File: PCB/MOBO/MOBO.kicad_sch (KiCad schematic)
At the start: 17 parts, among them J101 COMP_OUT, J102 COMP_5V, J103 COMP_GND, J104 RPi_GPio, J105 JST_02, J106 RPi_SDA0, J107 RPi_TV, J108 RPi_D-, J109 RPi_D+, J110 RPi_SCL0, J111 RPi_Ts5V, J112 RPi_TsGND

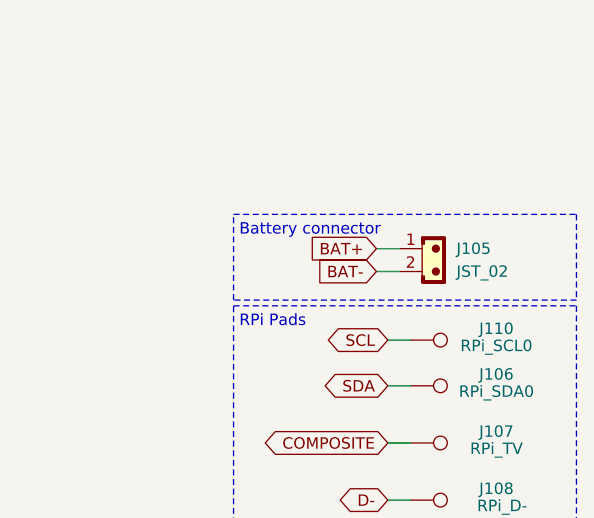
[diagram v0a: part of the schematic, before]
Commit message: fix: battery charging protection module
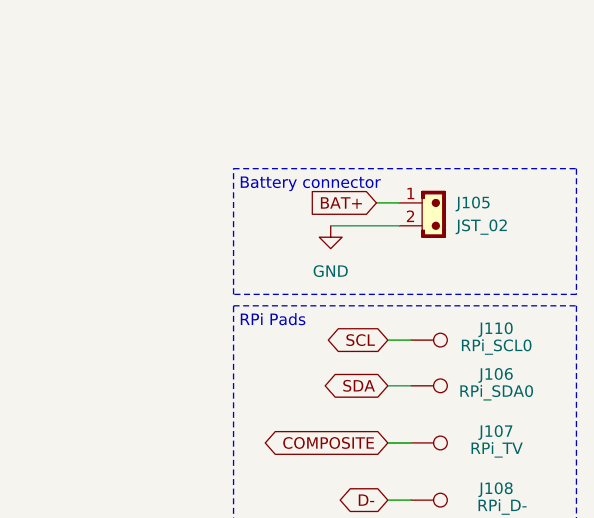
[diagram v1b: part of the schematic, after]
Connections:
- net BAT-: no longer J105.2
- net GND: now also J105.2
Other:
- moved on the sheet: J105
